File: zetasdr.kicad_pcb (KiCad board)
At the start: 2 copper layers, 77.5 x 43.5 mm, 47 parts, among them J2 USB_B, J5 Antenna, J6 AudioJack3_SwitchTR, Q1 BC547C, U1 74AHC1G04, U2 74HC74, U3 4052, U4 NE5532

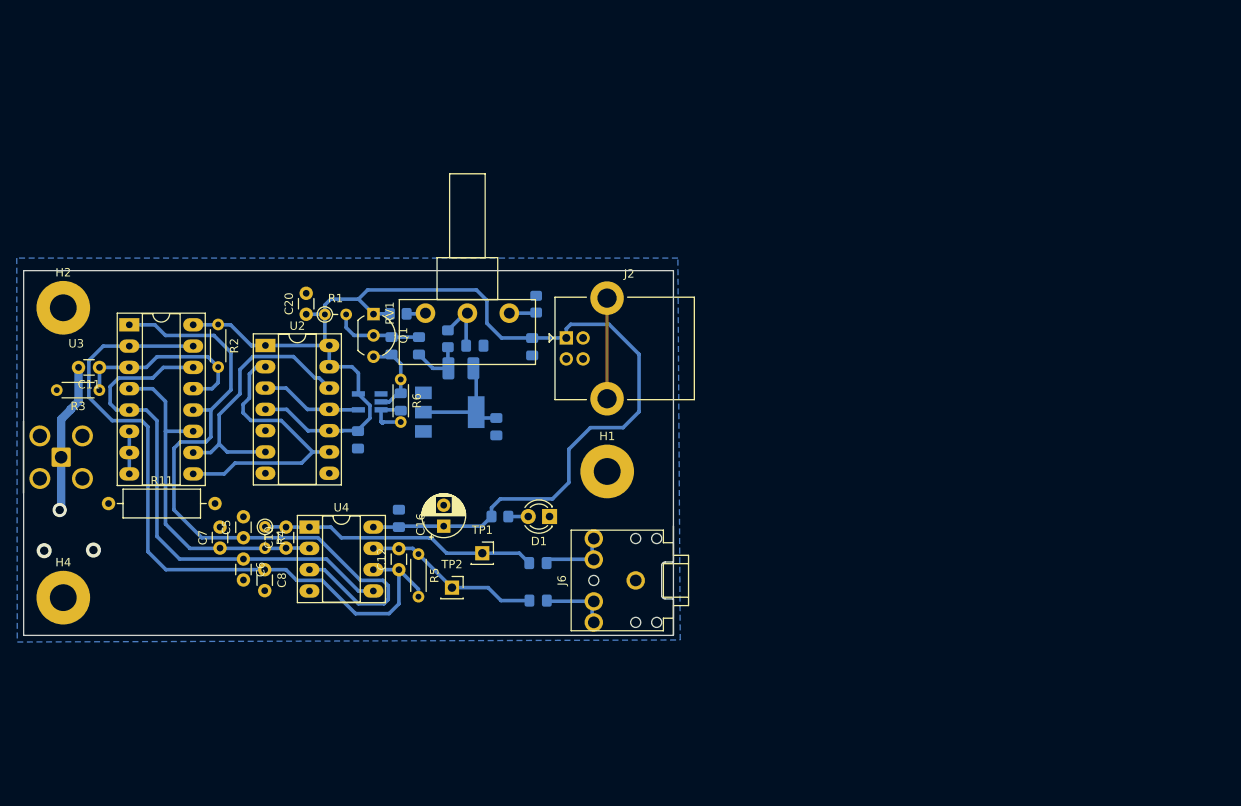
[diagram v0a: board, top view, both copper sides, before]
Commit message: first layout
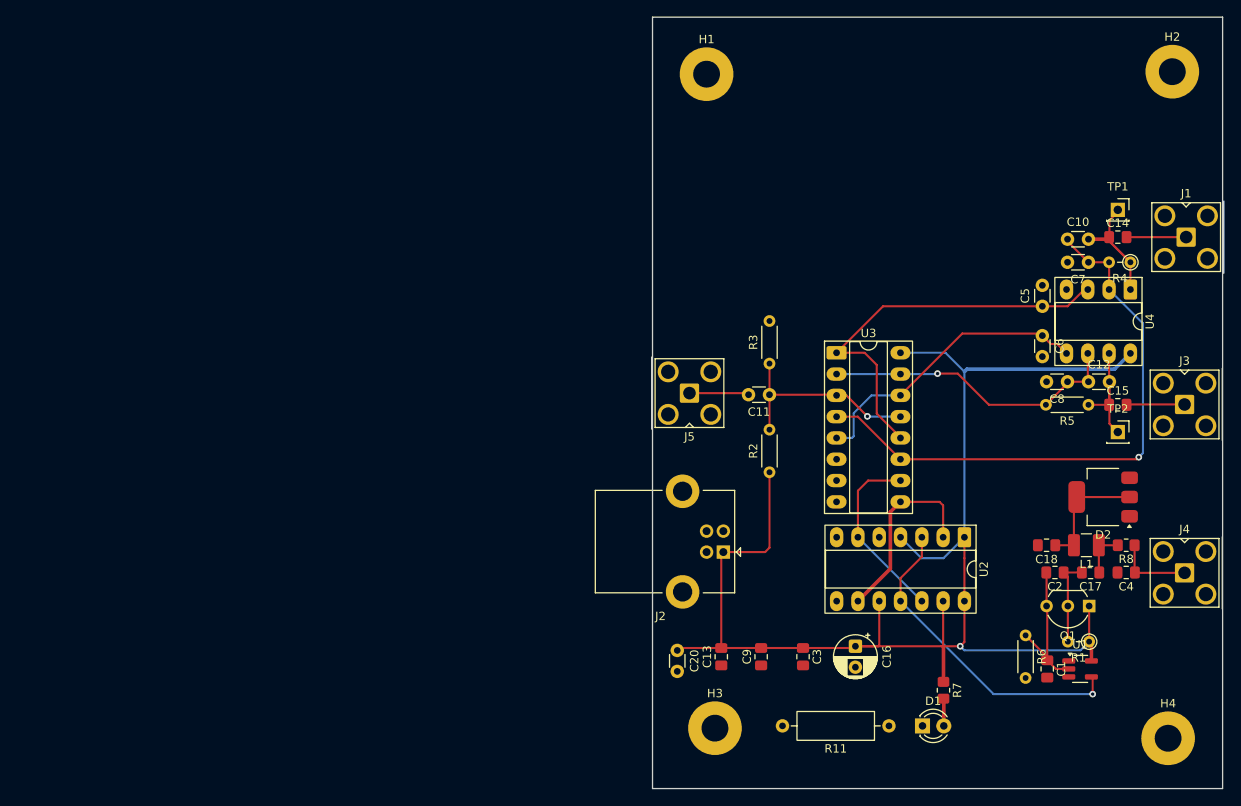
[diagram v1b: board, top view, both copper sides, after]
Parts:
- removed J6: AudioJack3_SwitchTR, Connector_Audio:Jack_3.5mm_CUI_SJ1-3525N_Horizontal
- removed R10, R9: 4k7, Resistor_SMD:R_0805_2012Metric_Pad1.20x1.40mm_HandSolder
- removed RV1: 50k, Potentiometer_THT:Potentiometer_Piher_T-16H_Single_Horizontal
- added H3: MountingHole_Pad, MountingHole:MountingHole_3.2mm_M3_Pad, F.Cu at (165.0, 138.6)
- added J1: Output I, Connector_Coaxial:SMA_Amphenol_901-143_Horizontal, F.Cu at (221.2, 80.0)
- added J3: Output Q, Connector_Coaxial:SMA_Amphenol_901-143_Horizontal, F.Cu at (221.0, 100.0)
- added J4: Input AWG, Connector_Coaxial:SMA_Amphenol_901-143_Horizontal, F.Cu at (221.0, 120.0)
- C1, C13, C14, C15, C17, C18, C2, C3, C4, C9, D2, J5, L1, R7, R8, U1: moved to F.Cu
- moved H2 135.2 mm to (219.5, 60.3)
- moved H4 132.8 mm to (219.0, 139.8)
- moved C7 109.0 mm to (209.5, 83.0), turned to 180 degrees
- moved R4 107.9 mm to (214.5, 83.0), turned to 180 degrees
- moved U4 101.9 mm to (214.5, 86.2), turned to -90 degrees
- moved C10 100.2 mm to (207.0, 80.2), turned to 0 degrees
- moved C5 99.2 mm to (204.0, 88.2)
- moved R1 99.2 mm to (209.6, 128.2), turned to 180 degrees
- moved C6 98.9 mm to (204.0, 91.8)
- moved C8 98.3 mm to (207.0, 97.2), turned to 180 degrees
- moved R11 96.8 mm to (185.7, 138.3), turned to 180 degrees
- moved Q1 92.2 mm to (209.6, 124.0), turned to 180 degrees
- moved U1 90.5 mm to (208.5, 131.5), turned to 0 degrees
- moved U2 86.4 mm to (194.7, 115.8), turned to -90 degrees
- moved TP1 86.2 mm to (213.0, 76.8)
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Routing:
- net Net-(U3-X2): track 85.7 -> 36.3 mm, vias 0 -> 1
- net Net-(U3-X0): track 81.2 -> 48.4 mm
- net Net-(U3-X3): track 41.5 -> 69.6 mm, vias 0 -> 1
- net Net-(U3-X1): track 61.6 -> 35.2 mm
- net Net-(U2A-C): track 12.2 -> 38.3 mm, vias 0 -> 1
- net VCC: track 147.5 -> 172.8 mm, vias 0 -> 1
- net GND: track 23.4 -> 0.00 mm, vias 2 -> 0
- net Net-(C10-Pad2): track 33.3 -> 17.6 mm
- net Net-(U2A-D): track 34.7 -> 23.0 mm
- net Net-(J5-In): track 18.2 -> 7.12 mm, vias 1 -> 0
- net Net-(U2A-~{Q}): track 32.2 -> 21.9 mm
- net Net-(Q1-E): track 10.1 -> 17.5 mm
- net Net-(C12-Pad2): track 21.2 -> 15.0 mm
- net Net-(R10-Pad1): track 3.34 -> 0.00 mm
- net Net-(J4-In): track 6.64 -> 9.20 mm
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- removed copper zone on B.Cu, net GND
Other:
- board size 77.5 x 43.5 mm -> 68 x 92 mm
